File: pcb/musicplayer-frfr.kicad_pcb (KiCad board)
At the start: 2 copper layers, 61.2 x 78.2 mm, 23 parts, among them J1 Battery, J2 AudioPlug3, J3 Display, SW1 SW_Push, SW2 SW_Push, SW3 SW_Push, SW4 RotaryEncoder_Switch, SW5 SW_SPDT, U1 XIAO-RP2350-SMD, U2 TP4056-42-ESOP8, U3 DFPLAYER_MINI

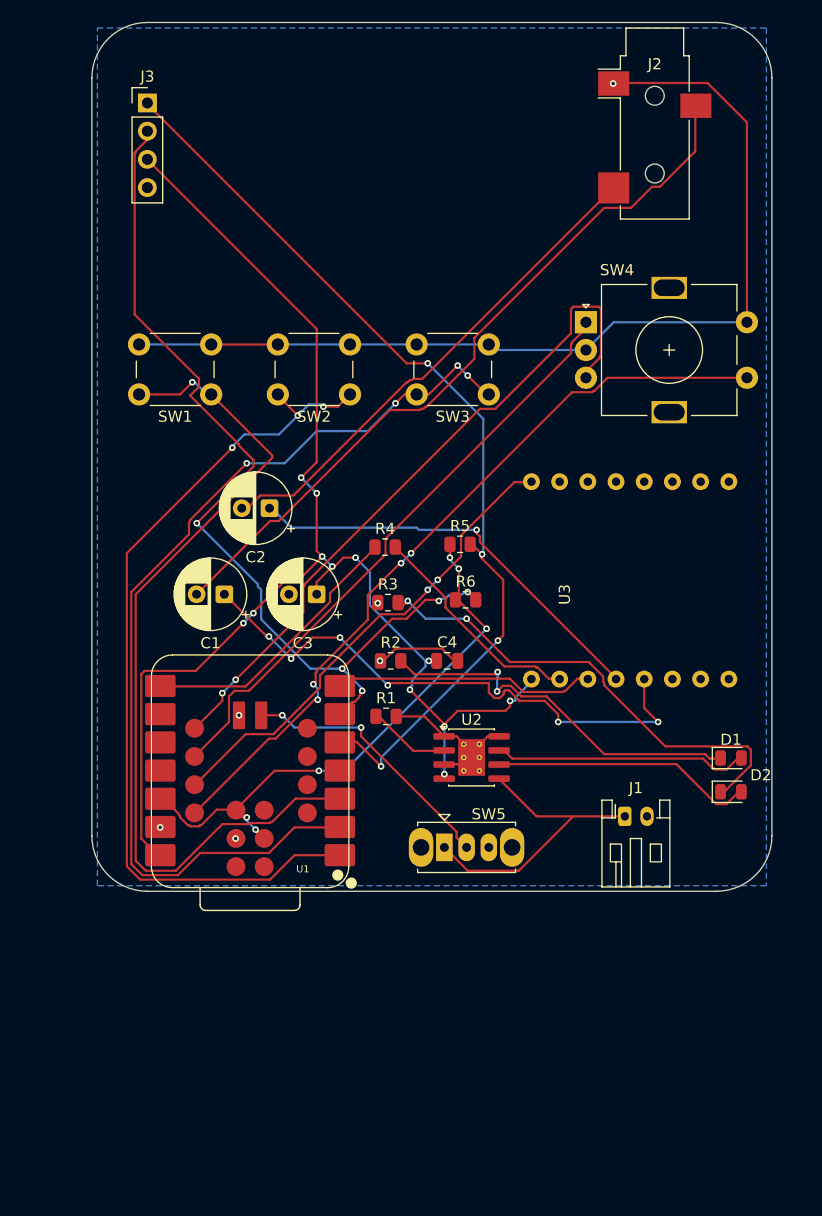
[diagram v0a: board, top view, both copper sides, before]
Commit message: layout pcb
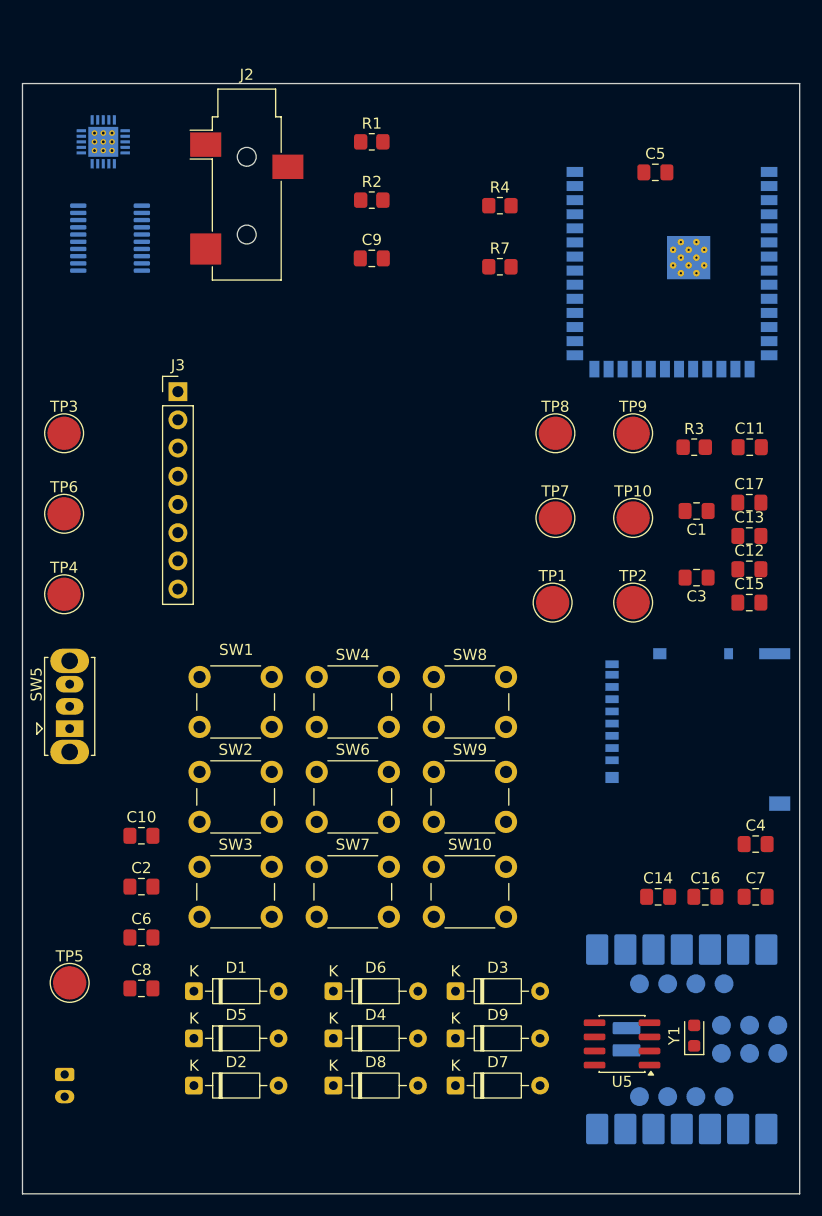
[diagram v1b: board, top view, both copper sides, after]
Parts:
- removed R5, R6: 4.7k, Resistor_SMD:R_0805_2012Metric
- added C10: 1uF, Capacitor_SMD:C_0805_2012Metric_Pad1.18x1.45mm_HandSolder, F.Cu at (110.7, 107.8)
- added C11: 1uF, Capacitor_SMD:C_0805_2012Metric_Pad1.18x1.45mm_HandSolder, F.Cu at (165.5, 72.8)
- added C12: 1uF, Capacitor_SMD:C_0805_2012Metric_Pad1.18x1.45mm_HandSolder, F.Cu at (165.5, 83.8)
- added C13: 0.1u, Capacitor_SMD:C_0805_2012Metric_Pad1.18x1.45mm_HandSolder, F.Cu at (165.5, 80.8)
- added C14: 10u, Capacitor_SMD:C_0805_2012Metric_Pad1.18x1.45mm_HandSolder, F.Cu at (157.2, 113.2)
- added C15: 10u, Capacitor_SMD:C_0805_2012Metric_Pad1.18x1.45mm_HandSolder, F.Cu at (165.5, 86.8)
- added C16: 10u, Capacitor_SMD:C_0805_2012Metric_Pad1.18x1.45mm_HandSolder, F.Cu at (161.5, 113.2)
- added C17: 10u, Capacitor_SMD:C_0805_2012Metric_Pad1.18x1.45mm_HandSolder, F.Cu at (165.5, 77.8)
- added C5: 2.2uF, Capacitor_SMD:C_0805_2012Metric_Pad1.18x1.45mm_HandSolder, F.Cu at (157.0, 48.0)
- added C6: 100nF, Capacitor_SMD:C_0805_2012Metric_Pad1.18x1.45mm_HandSolder, F.Cu at (110.7, 116.9)
- added C7: 10uF, Capacitor_SMD:C_0805_2012Metric_Pad1.18x1.45mm_HandSolder, F.Cu at (166.0, 113.2)
- added C8: 2.2nF, Capacitor_SMD:C_0805_2012Metric_Pad1.18x1.45mm_HandSolder, F.Cu at (110.7, 121.5)
- added C9: 2.2nF, Capacitor_SMD:C_0805_2012Metric_Pad1.18x1.45mm_HandSolder, F.Cu at (131.5, 55.8)
- added D3: 1N4149, Diode_THT:D_DO-35_SOD27_P7.62mm_Horizontal, F.Cu at (139.0, 121.8)
- added D4: 1N4149, Diode_THT:D_DO-35_SOD27_P7.62mm_Horizontal, F.Cu at (128.0, 126.0)
- added D5: 1N4149, Diode_THT:D_DO-35_SOD27_P7.62mm_Horizontal, F.Cu at (115.4, 126.0)
- added D6: 1N4149, Diode_THT:D_DO-35_SOD27_P7.62mm_Horizontal, F.Cu at (128.0, 121.8)
- added D7: 1N4149, Diode_THT:D_DO-35_SOD27_P7.62mm_Horizontal, F.Cu at (139.0, 130.2)
- added D8: 1N4149, Diode_THT:D_DO-35_SOD27_P7.62mm_Horizontal, F.Cu at (128.0, 130.2)
- added D9: 1N4149, Diode_THT:D_DO-35_SOD27_P7.62mm_Horizontal, F.Cu at (139.0, 126.0)
- added J4: Micro_SD_Card_Det1, Connector_Card:microSD_HC_Hirose_DM3AT-SF-PEJM5, B.Cu at (160.8, 98.2)
- added R7: 4.7k, Resistor_SMD:R_0805_2012Metric_Pad1.20x1.40mm_HandSolder, F.Cu at (143.0, 56.5)
- added SW10: Next, Button_Switch_THT:SW_PUSH_6mm, F.Cu at (137.1, 110.5)
- added SW6: Select, Button_Switch_THT:SW_PUSH_6mm, F.Cu at (126.5, 102.0)
- added SW7: Right, Button_Switch_THT:SW_PUSH_6mm, F.Cu at (126.5, 110.5)
- added SW8: Prev., Button_Switch_THT:SW_PUSH_6mm, F.Cu at (137.1, 93.5)
- added SW9: Down, Button_Switch_THT:SW_PUSH_6mm, F.Cu at (137.1, 102.0)
- added TP1: USB D-, TestPoint:TestPoint_Pad_D3.0mm, F.Cu at (147.8, 86.8)
- added TP10: ESP RX, TestPoint:TestPoint_Pad_D3.0mm, F.Cu at (155.0, 79.1)
- added TP2: USB D+, TestPoint:TestPoint_Pad_D3.0mm, F.Cu at (155.0, 86.8)
- added TP3: GND, TestPoint:TestPoint_Pad_D3.0mm, F.Cu at (103.8, 71.5)
- added TP4: +5V, TestPoint:TestPoint_Pad_D3.0mm, F.Cu at (103.8, 86.0)
- added TP5: VBAT, TestPoint:TestPoint_Pad_D3.0mm, F.Cu at (104.2, 121.0)
- added TP6: +3V3, TestPoint:TestPoint_Pad_D3.0mm, F.Cu at (103.8, 78.8)
- added TP7: ESP Boot, TestPoint:TestPoint_Pad_D3.0mm, F.Cu at (148.0, 79.1)
- added TP8: ESP Enable, TestPoint:TestPoint_Pad_D3.0mm, F.Cu at (148.0, 71.5)
- added TP9: ESP TX, TestPoint:TestPoint_Pad_D3.0mm, F.Cu at (155.0, 71.5)
- added U4: ESP32-S3-WROOM-1, RF_Module:ESP32-S3-WROOM-1, B.Cu at (158.5, 53.2)
- added U5: PCF8523T, Package_SO:SOIC-8_3.9x4.9mm_P1.27mm, F.Cu at (154.0, 126.5)
- added Y1: 32.768 kHz, Crystal:Crystal_SMD_2012-2Pin_2.0x1.2mm_HandSoldering, F.Cu at (160.5, 125.8)
- C1, C2: value 100u -> 100nF; footprint Capacitor_THT:CP_Radial_D6.3mm_P2.50mm -> Capacitor_SMD:C_0805_2012Metric_Pad1.18x1.45mm_HandSolder
- C3: value 100u -> 2.2uF; footprint Capacitor_THT:CP_Radial_D6.3mm_P2.50mm -> Capacitor_SMD:C_0805_2012Metric_Pad1.18x1.45mm_HandSolder
- C4: value 100n -> 100nF; footprint Capacitor_SMD:C_0805_2012Metric -> Capacitor_SMD:C_0805_2012Metric_Pad1.18x1.45mm_HandSolder
- D1, D2: value LED -> 1N4149; footprint LED_SMD:LED_0805_2012Metric -> Diode_THT:D_DO-35_SOD27_P7.62mm_Horizontal
- J1, U1: moved to B.Cu
- J3: footprint Connector_PinHeader_2.54mm:PinHeader_1x04_P2.54mm_Vertical -> Connector_PinHeader_2.54mm:PinHeader_1x08_P2.54mm_Vertical
- R1: value 2.4K -> 470; footprint Resistor_SMD:R_0805_2012Metric -> Resistor_SMD:R_0805_2012Metric_Pad1.20x1.40mm_HandSolder
- R2: value 1K -> 470; footprint Resistor_SMD:R_0805_2012Metric -> Resistor_SMD:R_0805_2012Metric_Pad1.20x1.40mm_HandSolder
- R3: value 1K -> 10k; footprint Resistor_SMD:R_0805_2012Metric -> Resistor_SMD:R_0805_2012Metric_Pad1.20x1.40mm_HandSolder
- R4: value 1K -> 4.7k; footprint Resistor_SMD:R_0805_2012Metric -> Resistor_SMD:R_0805_2012Metric_Pad1.20x1.40mm_HandSolder
- SW1: value SW_Push -> Vol Up
- SW2: value SW_Push -> Up
- SW3: value SW_Push -> Vol Down
- SW4: value RotaryEncoder_Switch -> Left; footprint Rotary_Encoder:RotaryEncoder_Alps_EC11E-Switch_Vertical_H20mm -> Button_Switch_THT:SW_PUSH_6mm
- SW5: value SW_SPDT -> SW_BAT
- U2: value TP4056-42-ESOP8 -> TPA6130A2RTJT; footprint Package_SO:SOIC-8-1EP_3.9x4.9mm_P1.27mm_EP2.41x3.3mm_ThermalVias -> footprints:RTJ20_2P7X2P7; moved to B.Cu
- U3: value DFPLAYER_MINI -> PCM5102; footprint DFPlayer:DFPlayer_V2 -> Package_SO:TSSOP-20_4.4x6.5mm_P0.65mm; moved to B.Cu
- moved U2 64.6 mm to (107.3, 45.2), turned to 180 degrees
- moved J1 55.5 mm to (103.8, 129.2), turned to -90 degrees
- moved D2 55.1 mm to (115.4, 130.2)
- moved D1 52.7 mm to (115.4, 121.8)
- moved R1 51.8 mm to (131.5, 45.2)
- moved SW3 49.9 mm to (116.0, 110.5), turned to 0 degrees
- moved U3 49.7 mm to (107.9, 53.9), turned to 180 degrees
- moved U1 45.8 mm to (159.4, 126.1), turned to 0 degrees
- moved C1 43.2 mm to (160.7, 78.5)
- moved R2 41.5 mm to (131.5, 50.5)
- moved SW4 40.1 mm to (126.5, 93.5)
- moved J2 37.2 mm to (120.2, 49.1)
- moved SW2 36.6 mm to (116.0, 102.0), turned to 0 degrees
- moved C2 36.0 mm to (110.7, 112.3), turned to 0 degrees
- moved SW5 35.4 mm to (104.2, 98.1), turned to 90 degrees
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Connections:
- net /NEXT renamed /COL3
- C1 pad 1: Net-(U3-DAC_L) -> Net-(U3-LDOO)
- C1 pad 2: /LEFT -> GND
- C2 pad 1: Net-(U3-DAC_R) -> GND
- C2 pad 2: /RIGHT -> +3V3
- C3 pad 1: /VBUS -> Net-(U3-CAPM)
- C3 pad 2: GND -> Net-(U3-CAPP)
- C4 pad 1: /VBUS -> GND
- C4 pad 2: GND -> +3V3
- D1 pad 1: Net-(D1-K) -> /ROW1
- D1 pad 2: /CHRG -> Net-(D1-A)
- D2 pad 1: Net-(D2-K) -> /ROW1
- D2 pad 2: /STDBY -> Net-(D2-A)
- J2 pad R: /LEFT -> /Audio/HPLEFT
- J2 pad T: /RIGHT -> /Audio/HPRIGHT
- J3 pad 1: /SDA -> /DISPLAY_LIGHT
- J3 pad 2: /SCL -> /DISPLAY_RST
- J3 pad 3: /VBUS -> /DISPLAY_DC
- J3 pad 4: GND -> /DISPLAY_CS
- R1 pad 1: Net-(U2-PROG) -> Net-(C9-Pad1)
- R1 pad 2: GND -> /Audio/OUTL
- R2 pad 1: GND -> Net-(C8-Pad2)
- R2 pad 2: Net-(D1-K) -> /Audio/OUTR
- R3 pad 1: GND -> +3V3
- R3 pad 2: Net-(D2-K) -> /ESP_BOOT
- R4 pad 1: /XIAO_TX -> +3V3
- R4 pad 2: Net-(U3-RX) -> /SDA
- SW1 pad 1: /BACK -> /COL1
- SW1 pad 2: GND -> Net-(D1-A)
- SW2 pad 1: /PLAY -> /COL2
- SW2 pad 2: GND -> Net-(D2-A)
- SW3 pad 2: GND -> Net-(D3-A)
- U1 pad 1: /PLAY -> /DISPLAY_RST
- U1 pad 10: unconnected-(U1-D9-Pad10) -> /SPI_MISO
- U1 pad 11: unconnected-(U1-D10-Pad11) -> /SPI_MOSI
- U1 pad 14: /VBUS -> +5V
- U1 pad 15: /ENCODER_SWITCH -> /DISPLAY_LIGHT
- U1 pad 16: /BUSY -> unconnected-(U1-D12-Pad16)
- U1 pad 17: /ENCODER_A -> /INTA
- U1 pad 18: /ENCODER_B -> /DISPLAY_CS
- U1 pad 19: unconnected-(U1-D15-Pad19) -> /COL2
- U1 pad 20: unconnected-(U1-D16-Pad20) -> /COL1
- U1 pad 21: unconnected-(U1-D17-Pad21) -> /ROW3
- U1 pad 22: unconnected-(U1-D18-Pad22) -> /ROW2
- U1 pad 3: /BACK -> /DISPLAY_DC
- U1 pad 4: unconnected-(U1-D3-Pad4) -> /SPI_CS
- U1 pad 7: /XIAO_RX -> /ESP_ENABLE
- U1 pad 8: /XIAO_TX -> /ROW1
- U1 pad 9: unconnected-(U1-D8-Pad9) -> /SPI_SCK
- U2 pad 1: GND -> /Audio/OUTL
- U2 pad 2: Net-(U2-PROG) -> GND
- U2 pad 4: /VBUS -> /Audio/OUTR
- U2 pad 5: /VBAT -> GND
- U2 pad 6: /STDBY -> /AMP_SDN
- U2 pad 7: /CHRG -> /SCL
- U2 pad 8: GND -> /SDA
- U3 pad 1: /VBUS -> +3V3
- U3 pad 11: unconnected-(U3-IO_2-Pad11) -> GND
- U3 pad 12: unconnected-(U3-ADKEY_1-Pad12) -> GND
- U3 pad 13: unconnected-(U3-ADKEY_2-Pad13) -> /I2S_BCK
- U3 pad 14: unconnected-(U3-USB+-Pad14) -> /I2S_DIN
- U3 pad 15: unconnected-(U3-USB--Pad15) -> /I2S_LRCK
- U3 pad 16: /BUSY -> GND
- U3 pad 2: Net-(U3-RX) -> Net-(U3-CAPP)
- U3 pad 3: /XIAO_RX -> GND
- U3 pad 4: Net-(U3-DAC_R) -> Net-(U3-CAPM)
- U3 pad 5: Net-(U3-DAC_L) -> /Audio/VNEG
- U3 pad 6: unconnected-(U3-SPK_1-Pad6) -> /Audio/OUTL
- U3 pad 7: GND -> /Audio/OUTR
- U3 pad 8: unconnected-(U3-SPK_2-Pad8) -> +3V3
- U3 pad 9: unconnected-(U3-IO_1-Pad9) -> GND
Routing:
- net /VBUS: track 123.6 -> 0.00 mm, vias 12 -> 0
- net GND: track 107.4 -> 0.00 mm, vias 7 -> 0
- net /COL3: track 87.8 -> 0.00 mm, vias 4 -> 0
- net /SDA: track 84.8 -> 0.00 mm, vias 4 -> 0
- net /SCL: track 84.3 -> 0.00 mm, vias 5 -> 0
- net /BACK: track 77.8 -> 0.00 mm, vias 1 -> 0
- net /PLAY: track 77.4 -> 0.00 mm, vias 3 -> 0
- net /ENCODER_SWITCH: track 69.1 -> 0.00 mm, vias 4 -> 0
- net /LEFT: track 66.7 -> 0.00 mm
- net /ENCODER_B: track 62.3 -> 0.00 mm, vias 2 -> 0
- net /ENCODER_A: track 54.5 -> 0.00 mm
- net Net-(U3-DAC_L): track 51.5 -> 0.00 mm, vias 6 -> 0
- net +3V3: track 51.1 -> 0.00 mm, vias 6 -> 0
- net /RIGHT: track 45.4 -> 0.00 mm
- net /BUSY: track 43.4 -> 0.00 mm, vias 2 -> 0
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- removed copper zone on B.Cu, net GND
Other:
- board size 61.2 x 78.2 mm -> 70 x 100 mm
- board text removed: "DISPLAY GOES HERE"
- board text removed: "made by avy for #hardware speedrun 18-20 Aug 2026"
